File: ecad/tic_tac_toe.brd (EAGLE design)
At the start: 85 x 54 mm, 37 parts, among them J1 PJ-102AH, U2 NCP1117ST50T3G, U3 ATMEGA8U2-AU, Y1 ECS-160-12-33-AGN-TR

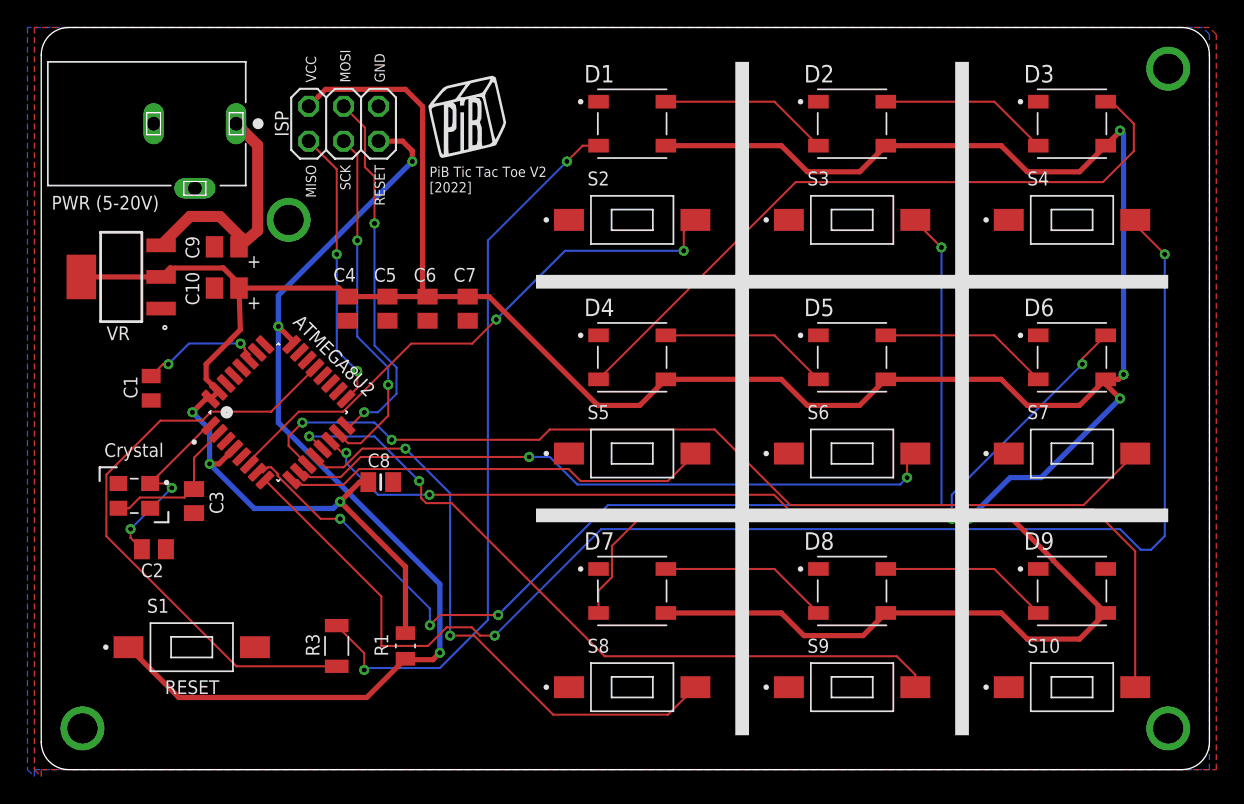
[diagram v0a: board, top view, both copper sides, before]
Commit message: ecad, gerbers
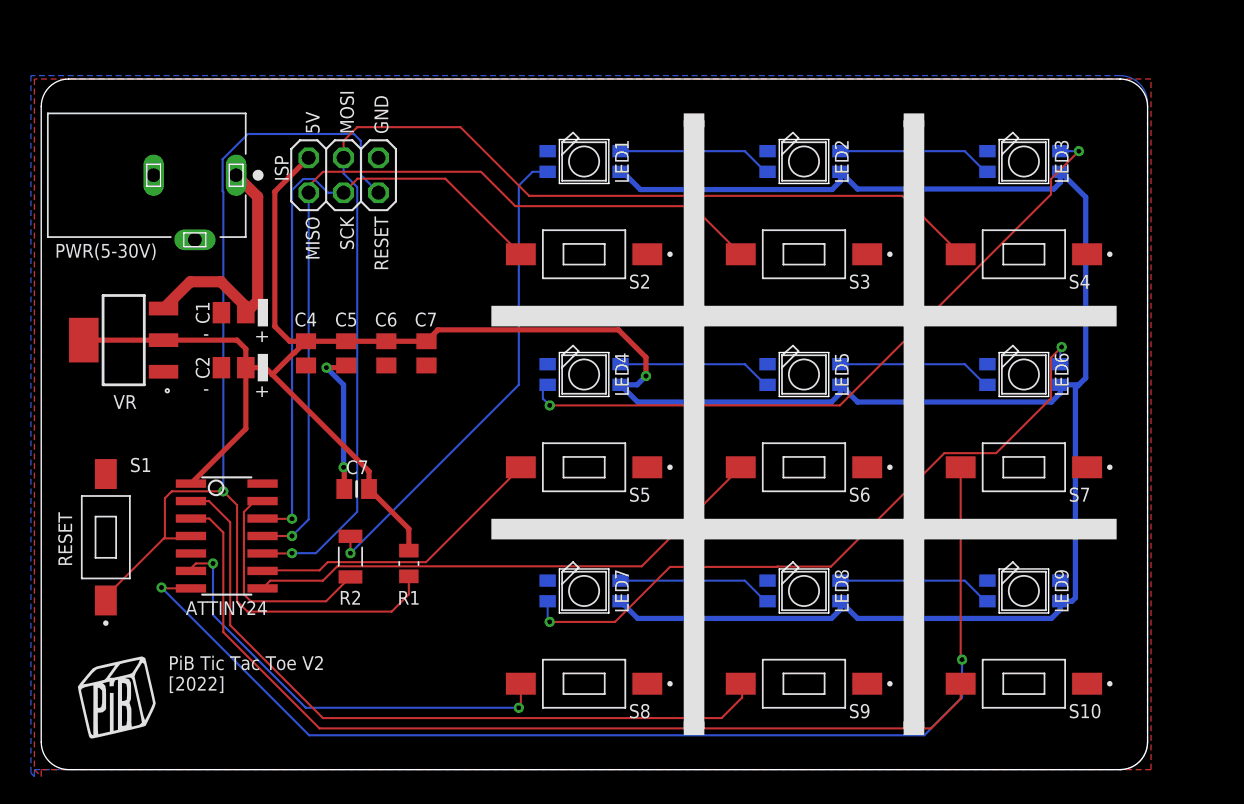
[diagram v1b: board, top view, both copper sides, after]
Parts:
- removed C10, C9: 10u, TAJR106M006R:CAPC2012X140N
- removed C11: 1u, GRM216R61E105KA12D:CAPC2012X70N
- removed C8: 4.7u, CL21A475KAQNNNE:CAPC2012X140N
- removed D1, D2, D3, D4, D5, D6, D7, D8, D9: 1655, 1655:LED_1655
- removed U2: NCP1117ST50T3G, NCP1117ST50T3G:SOT230P700X180-4N
- removed U3: ATMEGA8U2-AU, ATMEGA8U2-AU:QFP80P900X900X120-32N
- removed Y1: ECS-160-12-33-AGN-TR, ECS-160-12-33-AGN-TR:XTAL_ECS-160-12-33-AGN-TR
- added C1: 10u, TAJR106M006R (1):CAPC2012X140N
- added IC1: ATTINY24/44/84-SSU, attiny24_44_84:SOIC14
- added LED1, LED2, LED3, LED4, LED5, LED6, LED7, LED8, LED9: MICROBUILDER_WS2812B_SK6812E, Adafruit Slider Trinkey:MICROBUILDER_NEO3535_REVERSE
- added U1: NCP1117ST50T3G, NCP1117ST50T3G (1):SOT230P700X180-4N
- C2: value 22p -> 10u; device C0805C220J5GACTU:CAPC2012X140N -> TAJR106M006R (1):CAPC2012X140N
- C3: value 22p -> .1u; device C0805C220J5GACTU:CAPC2012X140N -> 08055F104K4T2A:CAPC2012X140N
- C7: value .1u -> 4.7u; device 08055F104K4T2A:CAPC2012X140N -> CL21A475KAQNNNE:CAPC2012X140N
- J1: value PJ-102AH -> Power_Jack
- JP1: value (none) -> ISP_Header
- S1: value 1437566-4 -> S_RESET
- moved U$1 49.3 mm to (5.50, 5.25)
- moved C7 15.4 mm to (22.9, 20.4), turned to 180 degrees
- moved C2 14.4 mm to (14.0, 29.2)
- moved C3 13.5 mm to (19.3, 30.3), turned to 90 degrees
- moved S1 10.2 mm to (4.70, 16.9), turned to 90 degrees
- moved R2 6.58 mm to (22.5, 15.5)
- moved R1 6.01 mm to (26.8, 15.0)
- moved S2 4.30 mm to (39.5, 37.5), turned to 180 degrees
- moved S3 4.30 mm to (55.5, 37.5), turned to 180 degrees
- moved S4 4.30 mm to (71.5, 37.5), turned to 180 degrees
- moved J1 3.75 mm to (7.68, 43.2)
- moved JP1 3.75 mm to (22.0, 43.2)
- moved S5 3.64 mm to (39.5, 22.0), turned to 180 degrees
- moved S6 3.64 mm to (55.5, 22.0), turned to 180 degrees
- moved S7 3.64 mm to (71.5, 22.0), turned to 180 degrees
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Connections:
- removed net IN_A: D1.2, R2.2
- removed net IN_B: D3.4, D4.2
- removed net IN_C: D6.4, D7.2
- removed net MISO: JP1.1, U3.17
- removed net MOSI: JP1.4, U3.16
- removed net N$1: R2.1, U3.21
- removed net N$8: C11.1, U3.27
- removed net SCK: JP1.3, U3.15
- removed net S_A: S2.2, U3.6
- removed net S_B: S3.2, U3.7
- removed net S_C: S4.2, U3.8
- removed net XTAL1: C2.1, U3.1, Y1.1
- removed net XTAL2: C3.1, U3.2, Y1.3
- new net IN: LED1.4-DIN, R2.2
- new net N$6: LED7.2-DOUT, LED8.4-DIN
- new net N$7: LED8.2-DOUT, LED9.4-DIN
- new net N$9: LED3.2-DOUT, LED4.4-DIN
- new net S_A/SCK: IC1.12, JP1.3, S2.2
- new net S_B/MISO: IC1.11, JP1.1, S3.2
- new net S_C/MOSI: IC1.10, JP1.4, S4.2
- net 5V: now also C2.2, C3.2, C7.1, IC1.1, LED1.1-VDD, LED2.1-VDD, LED3.1-VDD, LED4.1-VDD, LED5.1-VDD, LED6.1-VDD, LED7.1-VDD, LED8.1-VDD, LED9.1-VDD, U1.2, U1.4; no longer C10.2, C7.2, C8.1, D1.3, D2.3, D3.3, D4.3, D5.3, D6.3, D7.3, D8.3, D9.3, U2.2, U2.4, U3.31, U3.32, U3.4
- net GND: now also C1.1, C2.1, C3.1, C7.2, IC1.14, LED1.3-GND, LED2.3-GND, LED3.3-GND, LED4.3-GND, LED5.3-GND, LED6.3-GND, LED7.3-GND, LED8.3-GND, LED9.3-GND, U1.1; no longer C10.1, C11.2, C2.2, C3.2, C7.1, C8.2, C9.1, D1.1, D2.1, D3.1, D4.1, D5.1, D6.1, D7.1, D8.1, D9.1, U2.1, U3.28, U3.3, Y1.2, Y1.4
- net N$14: now also LED6.2-DOUT, LED7.4-DIN; no longer D1.4, D2.2
- net N$15: now also IC1.13, R2.1; no longer D7.4, D8.2
- net N$2: now also LED1.2-DOUT, LED2.4-DIN; no longer D2.4, D3.2
- net N$3: now also LED2.2-DOUT, LED3.4-DIN; no longer D4.4, D5.2
- net N$4: now also LED4.2-DOUT, LED5.4-DIN; no longer D5.4, D6.2
- net N$5: now also LED5.2-DOUT, LED6.4-DIN; no longer D8.4, D9.2
- net RESET: now also IC1.4; no longer U3.24
- net S_D: now also IC1.9; no longer U3.9
- net S_E: now also IC1.8; no longer U3.10
- net S_F: now also IC1.7; no longer U3.11
- net S_G: now also IC1.6; no longer U3.12
- net S_H: now also IC1.2; no longer U3.13
- net S_I: now also IC1.3; no longer U3.14
- net VCC: now also C1.2, U1.3; no longer C9.2, U2.3
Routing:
- net S_C: track 101.5 -> 0.00 mm, vias 2 -> 0
- net S_C/MOSI: track 0.00 -> 84.7 mm, vias 0 -> 1
- net S_B: track 80.7 -> 0.00 mm, vias 4 -> 0
- net S_B/MISO: track 0.00 -> 62.5 mm, vias 0 -> 1
- net IN_A: track 53.1 -> 0.00 mm, vias 2 -> 0
- net IN_B: track 50.5 -> 0.00 mm
- net N$9: track 0.00 -> 50.0 mm, vias 0 -> 2
- net IN_C: track 48.8 -> 0.00 mm, vias 2 -> 0
- net S_A/SCK: track 0.00 -> 46.2 mm, vias 0 -> 1
- net N$1: track 43.6 -> 0.00 mm
- net S_A: track 40.8 -> 0.00 mm, vias 2 -> 0
- net 5V: track 269.8 -> 230.6 mm, vias 7 -> 1
- net N$14: track 12.4 -> 50.1 mm, vias 0 -> 2
- net IN: track 0.00 -> 35.6 mm, vias 0 -> 1
- net MOSI: track 27.2 -> 0.00 mm, vias 2 -> 0
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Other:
- board size 85 x 54 mm -> 80.5 x 50.2 mm
- board text added: "-"
- board text added: "5V"
- board text added: "ATTINY24"
- board text added: "LED1"
- board text added: "LED2"
- board text added: "LED3"
- board text added: "LED4"
- board text added: "LED5"
- board text added: "LED6"
- board text added: "LED7"
- board text added: "LED8"
- board text added: "LED9"
- board text added: "PWR(5-30V)"
- board text added: "R2"
- board text removed: "ATMEGA8U2"
- board text removed: "C10"
- board text removed: "C3"
- board text removed: "C8"
- board text removed: "C9"
- board text removed: "Crystal"
- board text removed: "PWR (5-20V)"
- board text removed: "R3"
- board text removed: "VCC"
